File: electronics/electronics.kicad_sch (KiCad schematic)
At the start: 14 parts, among them J1 USB_C_Receptacle_USB2.0_14P, U1 ESP32-S3-WROOM-1, U3 NCP1117-3.3_SOT223, U5 NCP1117-3.3_SOT223

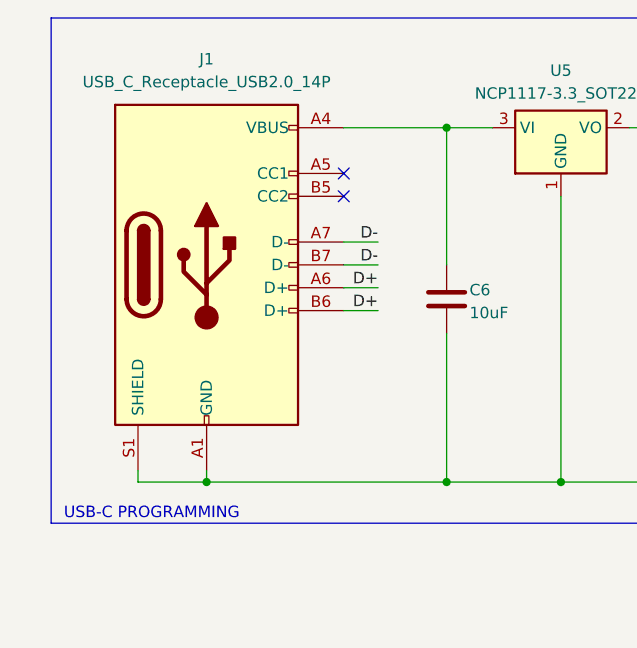
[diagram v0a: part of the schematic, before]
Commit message: BOM + Gerbers: Final Iteration (Hopefully)
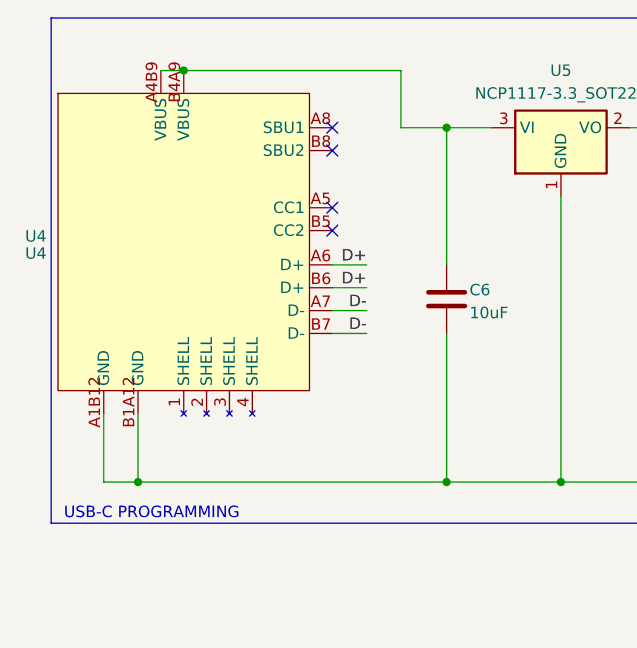
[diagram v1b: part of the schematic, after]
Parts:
- removed J1: USB_C_Receptacle_USB2.0_14P, Connector_USB:USB_C_Receptacle_GCT_USB4110, symbol Connector:USB_C_Receptacle_USB2.0_14P
- added U4: U4, Uni:USB-C-SMD_G-SWITCH_GT-USB-7010ASV, symbol USB-C:USB-C_Plug
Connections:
- net D+: now also U4.A6 (D+), U4.B6 (D+)
- net D-: now also U4.A7 (D-), U4.B7 (D-)
- net GND: now also U4.A1B12 (GND), U4.B1A12 (GND)
- net at C6.1, U5.3 (VI): now also U4.A4B9 (VBUS), U4.B4A9 (VBUS)
- no-connect marks 39 -> 41
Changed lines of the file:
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@@
+	)
+	(junction
+		(at 21.59 63.5)
+		(diameter 0)
+		(color 0 0 0 0)
 	)
 	(junction
@@
 	)
 	(junction
-		(at 55.88 63.5)
+		(at 26.67 17.78)
 		(diameter 0)
 		(color 0 0 0 0)
 	)
 	(junction
-		(at 29.21 63.5)
+		(at 55.88 63.5)
 		(diameter 0)
 		(color 0 0 0 0)
@@
 	)
 	(no_connect
-		(at 44.45 31.75)
+		(at 43.18 35.56)
 	)
 	(no_connect
@@
 	)
 	(no_connect
-		(at 44.45 29.21)
+		(at 43.18 24.13)
+	)
+	(no_connect
+		(at 43.18 33.02)
 	)
 	(no_connect
@@
 	)
 	(no_connect
+		(at 43.18 26.67)
+	)
+	(no_connect
 		(at 256.54 99.06)
 	)
@@
 	(wire
 		(pts
+			(xy 50.8 24.13) (xy 55.88 24.13)
+		)
+		(stroke
+			(width 0)
+			(type default)
+		)
+	)
+	(wire
+		(pts
 			(xy 269.24 138.43) (xy 269.24 139.7)
 		)
@@
 	(wire
 		(pts
-			(xy 29.21 63.5) (xy 29.21 62.23)
-		)
-		(stroke
-			(width 0)
-			(type default)
-		)
-	)
-	(wire
-		(pts
 			(xy 121.92 35.56) (xy 121.92 36.83)
 		)
@@
 	(wire
 		(pts
-			(xy 55.88 63.5) (xy 29.21 63.5)
+			(xy 17.78 63.5) (xy 21.59 63.5)
 		)
 		(stroke
@@
 	(wire
 		(pts
+			(xy 50.8 17.78) (xy 50.8 24.13)
+		)
+		(stroke
+			(width 0)
+			(type default)
+		)
+	)
+	(wire
+		(pts
 			(xy 107.95 20.32) (xy 114.3 20.32)
 		)
@@
 	(wire
 		(pts
+			(xy 21.59 55.88) (xy 21.59 63.5)
+		)
+		(stroke
+			(width 0)
+			(type default)
+		)
+	)
+	(wire
+		(pts
 			(xy 271.78 110.49) (xy 271.78 124.46)
 		)
@@
 	(wire
 		(pts
-			(xy 44.45 44.45) (xy 48.26 44.45)
+			(xy 43.18 39.37) (xy 46.99 39.37)
 		)
 		(stroke
@@
 	(wire
 		(pts
+			(xy 21.59 63.5) (xy 55.88 63.5)
+		)
+		(stroke
+			(width 0)
+			(type default)
+		)
+	)
+	(wire
+		(pts
 			(xy 123.19 82.55) (xy 123.19 85.09)
 		)
@@
 	(wire
 		(pts
-			(xy 44.45 39.37) (xy 48.26 39.37)
+			(xy 24.13 17.78) (xy 26.67 17.78)
+		)
+		(stroke
+			(width 0)
+			(type default)
+		)
+	)
+	(wire
+		(pts
+			(xy 43.18 44.45) (xy 46.99 44.45)
 		)
 		(stroke
@@
 	(wire
 		(pts
-			(xy 44.45 36.83) (xy 48.26 36.83)
+			(xy 43.18 46.99) (xy 46.99 46.99)
 		)
 		(stroke
@@
 	(wire
 		(pts
-			(xy 44.45 41.91) (xy 48.26 41.91)
+			(xy 43.18 41.91) (xy 46.99 41.91)
 		)
 		(stroke
@@
 	(wire
 		(pts
-			(xy 44.45 24.13) (xy 55.88 24.13)
+			(xy 17.78 55.88) (xy 17.78 63.5)
 		)
 		(stroke
@@
 	(wire
 		(pts
+			(xy 26.67 17.78) (xy 50.8 17.78)
+		)
+		(stroke
+			(width 0)
+			(type default)
+		)
+	)
+	(wire
+		(pts
 			(xy 107.95 35.56) (xy 121.92 35.56)
 		)
@@
 	(wire
 		(pts
-			(xy 21.59 62.23) (xy 21.59 63.5)
-		)
-		(stroke
-			(width 0)
-			(type default)
-		)
-	)
-	(wire
-		(pts
 			(xy 55.88 24.13) (xy 60.96 24.13)
 		)
@@
 		(pts
 			(xy 96.52 20.32) (xy 96.52 35.56)
-		)
-		(stroke
-			(width 0)
-			(type default)
-		)
-	)
-	(wire
-		(pts
-			(xy 21.59 63.5) (xy 29.21 63.5)
 		)
 		(stroke
@@
 	)
 	(label "D-"
-		(at 48.26 39.37 180)
+		(at 46.99 44.45 180)
 		(effects
 			(font
@@
 	)
 	(label "D+"
-		(at 48.26 41.91 180)
+		(at 46.99 41.91 180)
 		(effects
 			(font
@@
 	)
 	(label "D-"
-		(at 48.26 36.83 180)
+		(at 46.99 46.99 180)
 		(effects
 			(font
@@
 	)
 	(label "D+"
-		(at 48.26 44.45 180)
+		(at 46.99 39.37 180)
 		(effects
 			(font
@@
 				(path "/d89b62dc-8d2d-44ba-babc-ef0071540948"
 					(reference "C1")
-					(unit 1)
-				)
-			)
-		)
-	)
-	(symbol
-		(lib_id "Connector:USB_C_Receptacle_USB2.0_14P")
-		(at 29.21 39.37 0)
-		(unit 1)
-		(exclude_from_sim no)
-		(in_bom yes)
-		(on_board yes)
-		(dnp no)
-		(fields_autoplaced yes)
-		(property "Reference" "J1"
-			(at 29.21 16.51 0)
-			(effects
-				(font
-					(size 1.27 1.27)
-				)
-			)
-		)
-		(property "Value" "USB_C_Receptacle_USB2.0_14P"
-			(at 29.21 19.05 0)
-			(effects
-				(font
-					(size 1.27 1.27)
-				)
-			)
-		)
-		(property "Footprint" "Connector_USB:USB_C_Receptacle_GCT_USB4110"
-			(at 33.02 39.37 0)
-			(effects
-				(font
-					(size 1.27 1.27)
-				)
-				(hide yes)
-			)
-		)
-		(property "Datasheet" "https://www.usb.org/sites/default/files/documents/usb_type-c.zip"
-			(at 33.02 39.37 0)
-			(effects
-				(font
-					(size 1.27 1.27)
-				)
-				(hide yes)
-			)
-		)
-		(property "Description" "USB 2.0-only 14P Type-C Receptacle connector"
-			(at 29.21 39.37 0)
-			(effects
-				(font
-					(size 1.27 1.27)
-				)
-				(hide yes)
-			)
-		)
-		(pin "B12"
-		)
-		(pin "B6"
-		)
-		(pin "S1"
-		)
-		(pin "B4"
-		)
-		(pin "A9"
-		)
-		(pin "B5"
-		)
-		(pin "B1"
-		)
-		(pin "B7"
-		)
-		(pin "B9"
-		)
-		(pin "A7"
-		)
-		(pin "A4"
-		)
-		(pin "A5"
-		)
-		(pin "A12"
-		)
-		(pin "A1"
-		)
-		(pin "A6"
-		)
-		(instances
-			(project "electronics"
-				(path "/d89b62dc-8d2d-44ba-babc-ef0071540948"
-					(reference "J1")
 					(unit 1)
 				)
@@
 					(unit 1)
 				)
+			)
+		)
+	)
+	(symbol
+		(lib_id "USB-C:USB-C_Plug")
+		(at 12.7 53.34 0)
+		(unit 1)
+		(exclude_from_sim no)
+		(in_bom yes)
+		(on_board yes)
+		(dnp no)
+		(fields_autoplaced yes)
+		(property "Reference" "U4"
+			(at 11.43 36.1949 0)
+			(effects
+				(font
+					(size 1.27 1.27)
+				)
+				(justify right)
+			)
+		)
+		(property "Value" "U4"
+			(at 11.43 38.1 0)
+			(effects
+				(font
+					(size 1.27 1.27)
+				)
+				(justify right)
+			)
+		)
+		(property "Footprint" "Uni:USB-C-SMD_G-SWITCH_GT-USB-7010ASV"
+			(at 2.54 58.928 0)
+			(effects
+				(font
+					(size 1.27 1.27)
+				)
+				(hide yes)
+			)
+		)
+		(property "Datasheet" ""
+			(at 2.54 58.928 0)
+			(effects
+				(font
+					(size 1.27 1.27)
+				)
+				(hide yes)
+			)
+		)
+		(property "Description" ""
+			(at 2.54 58.928 0)
+			(effects
+				(font
+					(size 1.27 1.27)
+				)
+				(hide yes)
+			)
+		)
+		(pin "B5"
+		)
+		(pin "A8"
+		)
+		(pin "A7"
+		)
+		(pin "B6"
+		)
+		(pin "B8"
+		)
+		(pin "A6"
+		)
+		(pin "1"
+		)
+		(pin "4"
+		)
+		(pin "3"
+		)
+		(pin "2"
+		)
+		(pin "B1A12"
+		)
+		(pin "A5"
+		)
+		(pin "B7"
+		)
+		(pin "A1B12"
+		)
+		(pin "A4B9"
+		)
+		(pin "B4A9"
+		)
+		(instances
+			(project ""
+				(path "/d89b62dc-8d2d-44ba-babc-ef0071540948"
+					(reference "U4")
+					(unit 1)
+				)

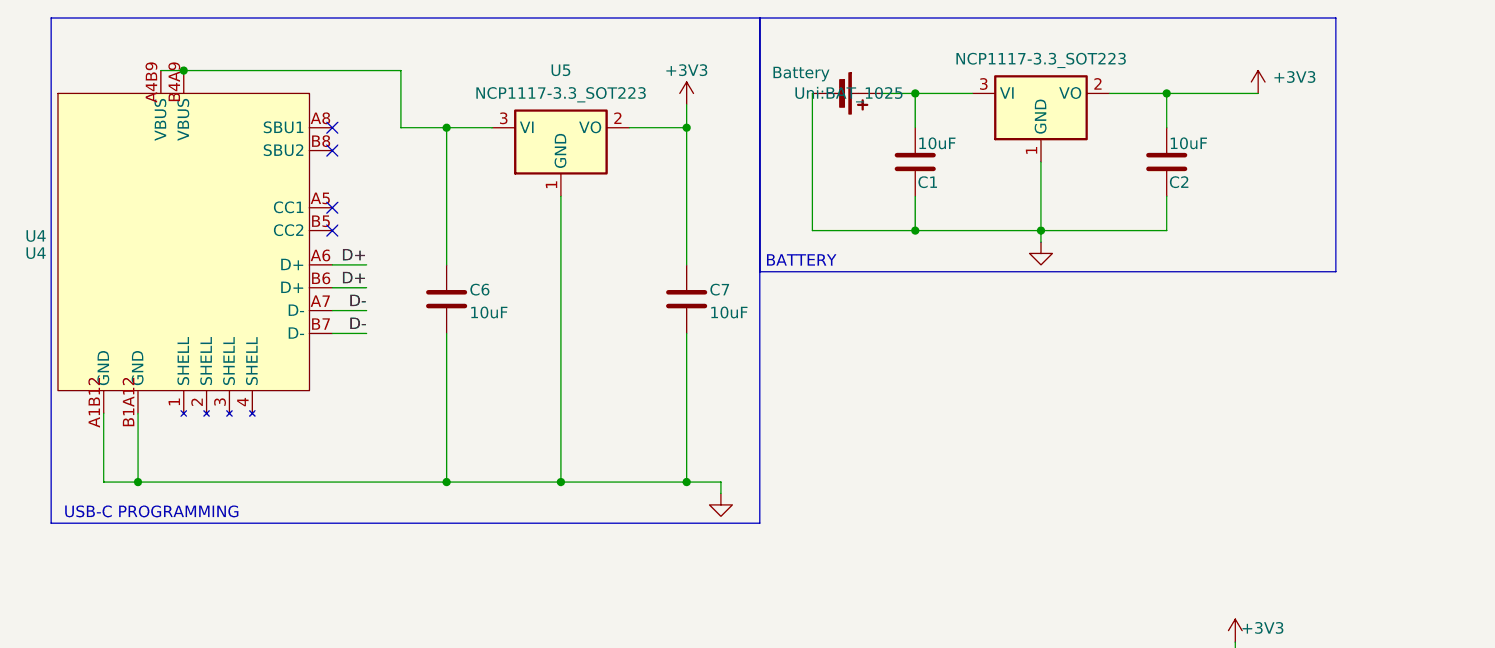
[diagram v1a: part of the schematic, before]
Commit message: BOM + Gerbers: Final Iteration (Hopefully)
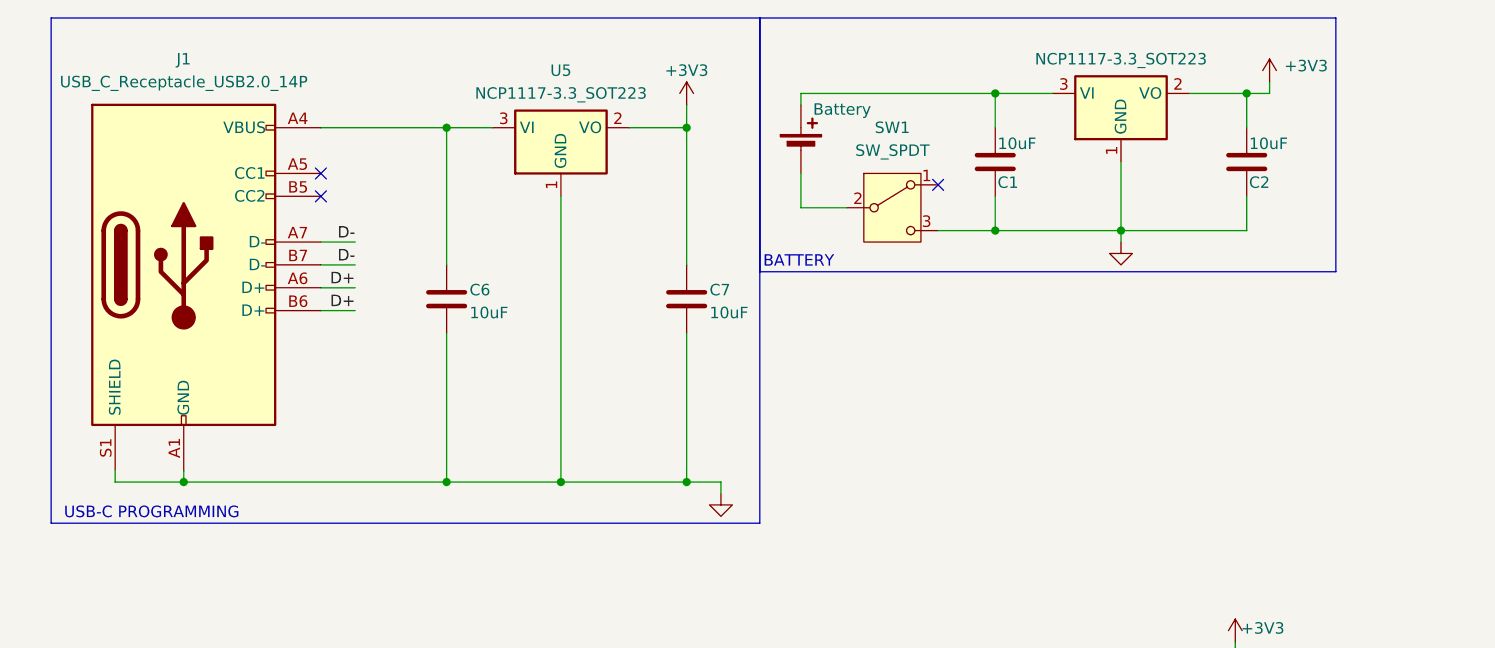
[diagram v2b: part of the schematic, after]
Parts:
- removed U4: U4, Uni:USB-C-SMD_G-SWITCH_GT-USB-7010ASV, symbol USB-C:USB-C_Plug
- added J1: USB_C_Receptacle_USB2.0_14P, Connector_USB:USB_C_Receptacle_GCT_USB4110, symbol Connector:USB_C_Receptacle_USB2.0_14P
- added SW1: SW_SPDT, Uni:CUS-12TB_NDC, symbol Switch:SW_SPDT
- BT1: footprint Uni:BAT_1025 -> Uni:BAT_3024-2
- R1: footprint Resistor_SMD:R_0402_1005Metric -> Resistor_SMD:R_0603_1608Metric
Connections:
- net D+: now also J1.A6 (D+), J1.B6 (D+)
- net D-: now also J1.A7 (D-), J1.B7 (D-)
- net GND: now also J1.A1 (GND), J1.A12 (GND), J1.B1 (GND), J1.B12 (GND), J1.S1 (SHIELD), SW1.3 (C); no longer BT1.2 (-)
- net at C6.1, U5.3 (VI): now also J1.A4 (VBUS), J1.A9 (VBUS), J1.B4 (VBUS), J1.B9 (VBUS)
- new net: BT1.2 (-), SW1.2 (B)
- no-connect marks 41 -> 40
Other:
- moved on the sheet: C1, C2
